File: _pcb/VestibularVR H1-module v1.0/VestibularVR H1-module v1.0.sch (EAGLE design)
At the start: 52 parts, among them IC1 FT232RL, IC2 74LVC1G07DBV, IC4 74LVC1G07DBV, IC5 74LVC1G07DBV, IC6 74LVC1G07DBV

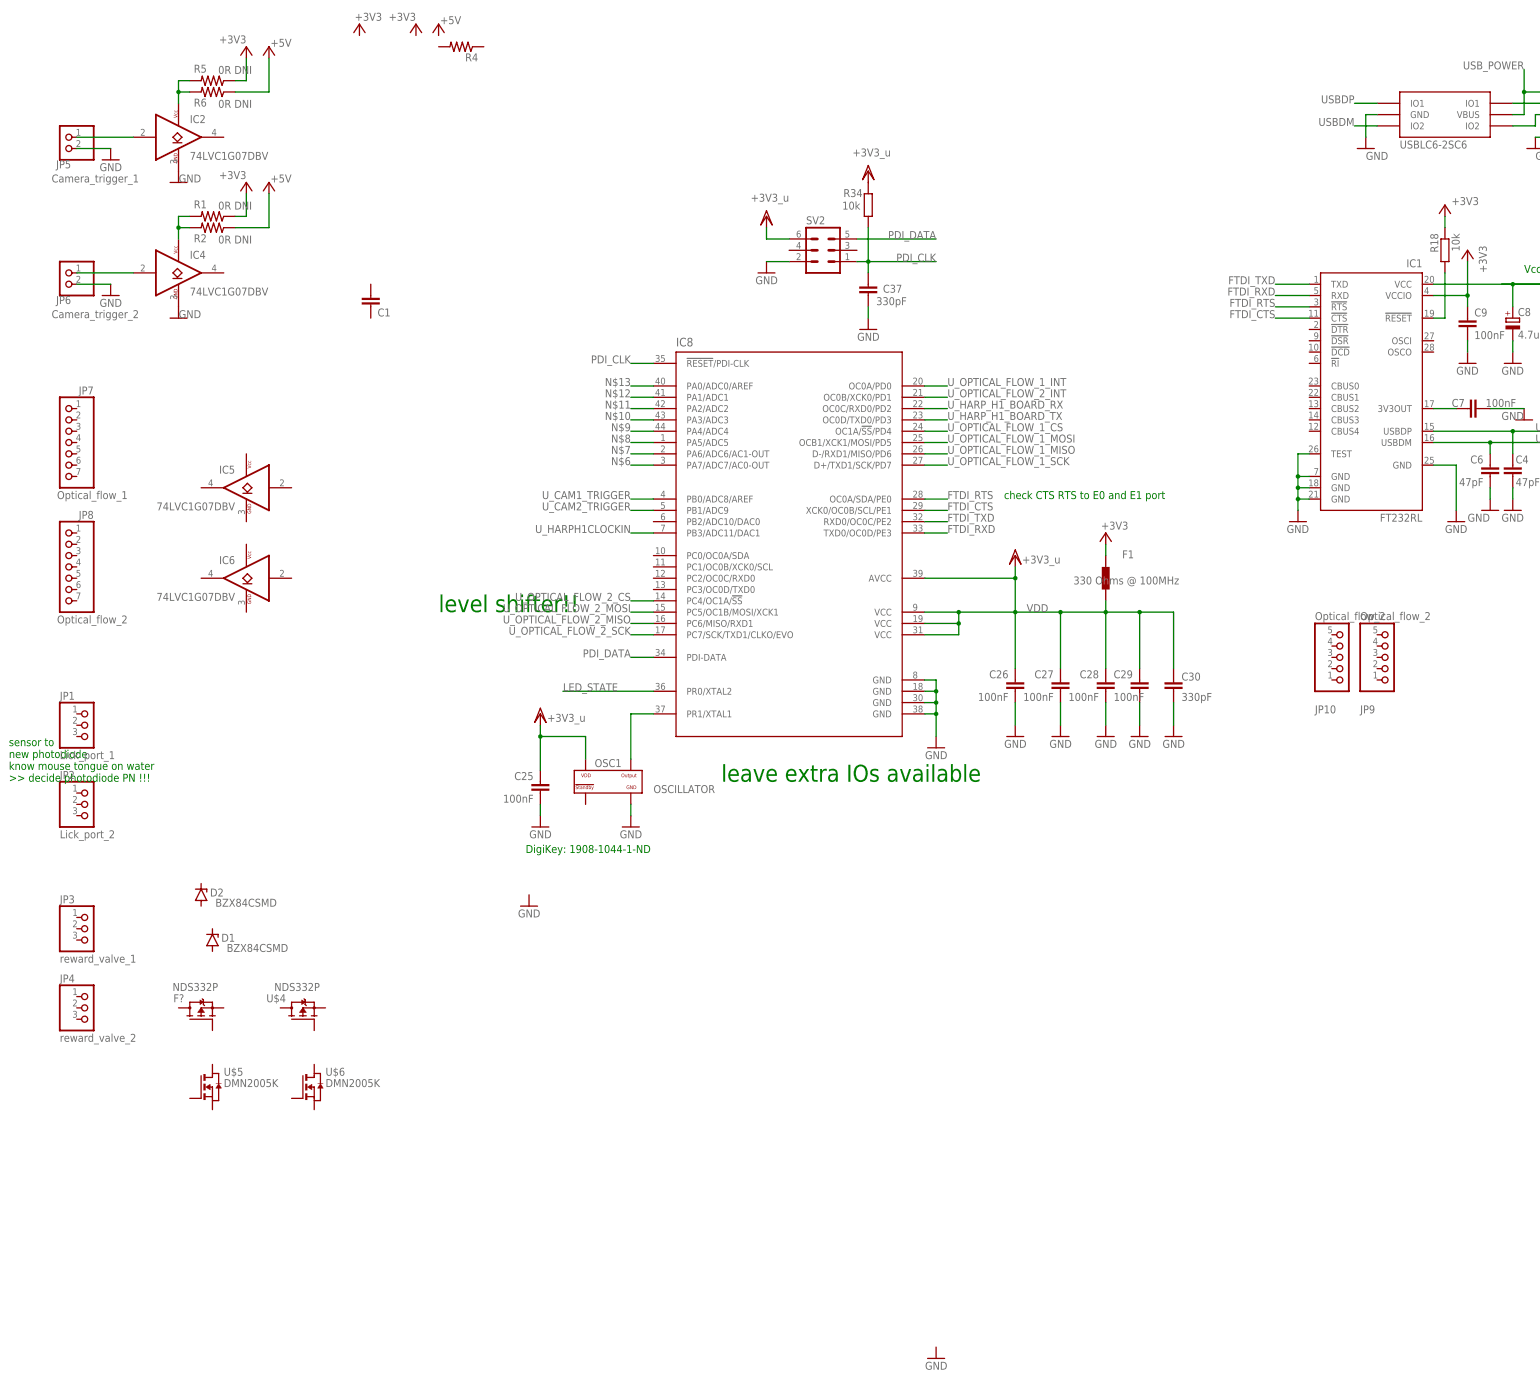
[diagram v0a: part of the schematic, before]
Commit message: pcb v1.0 developed
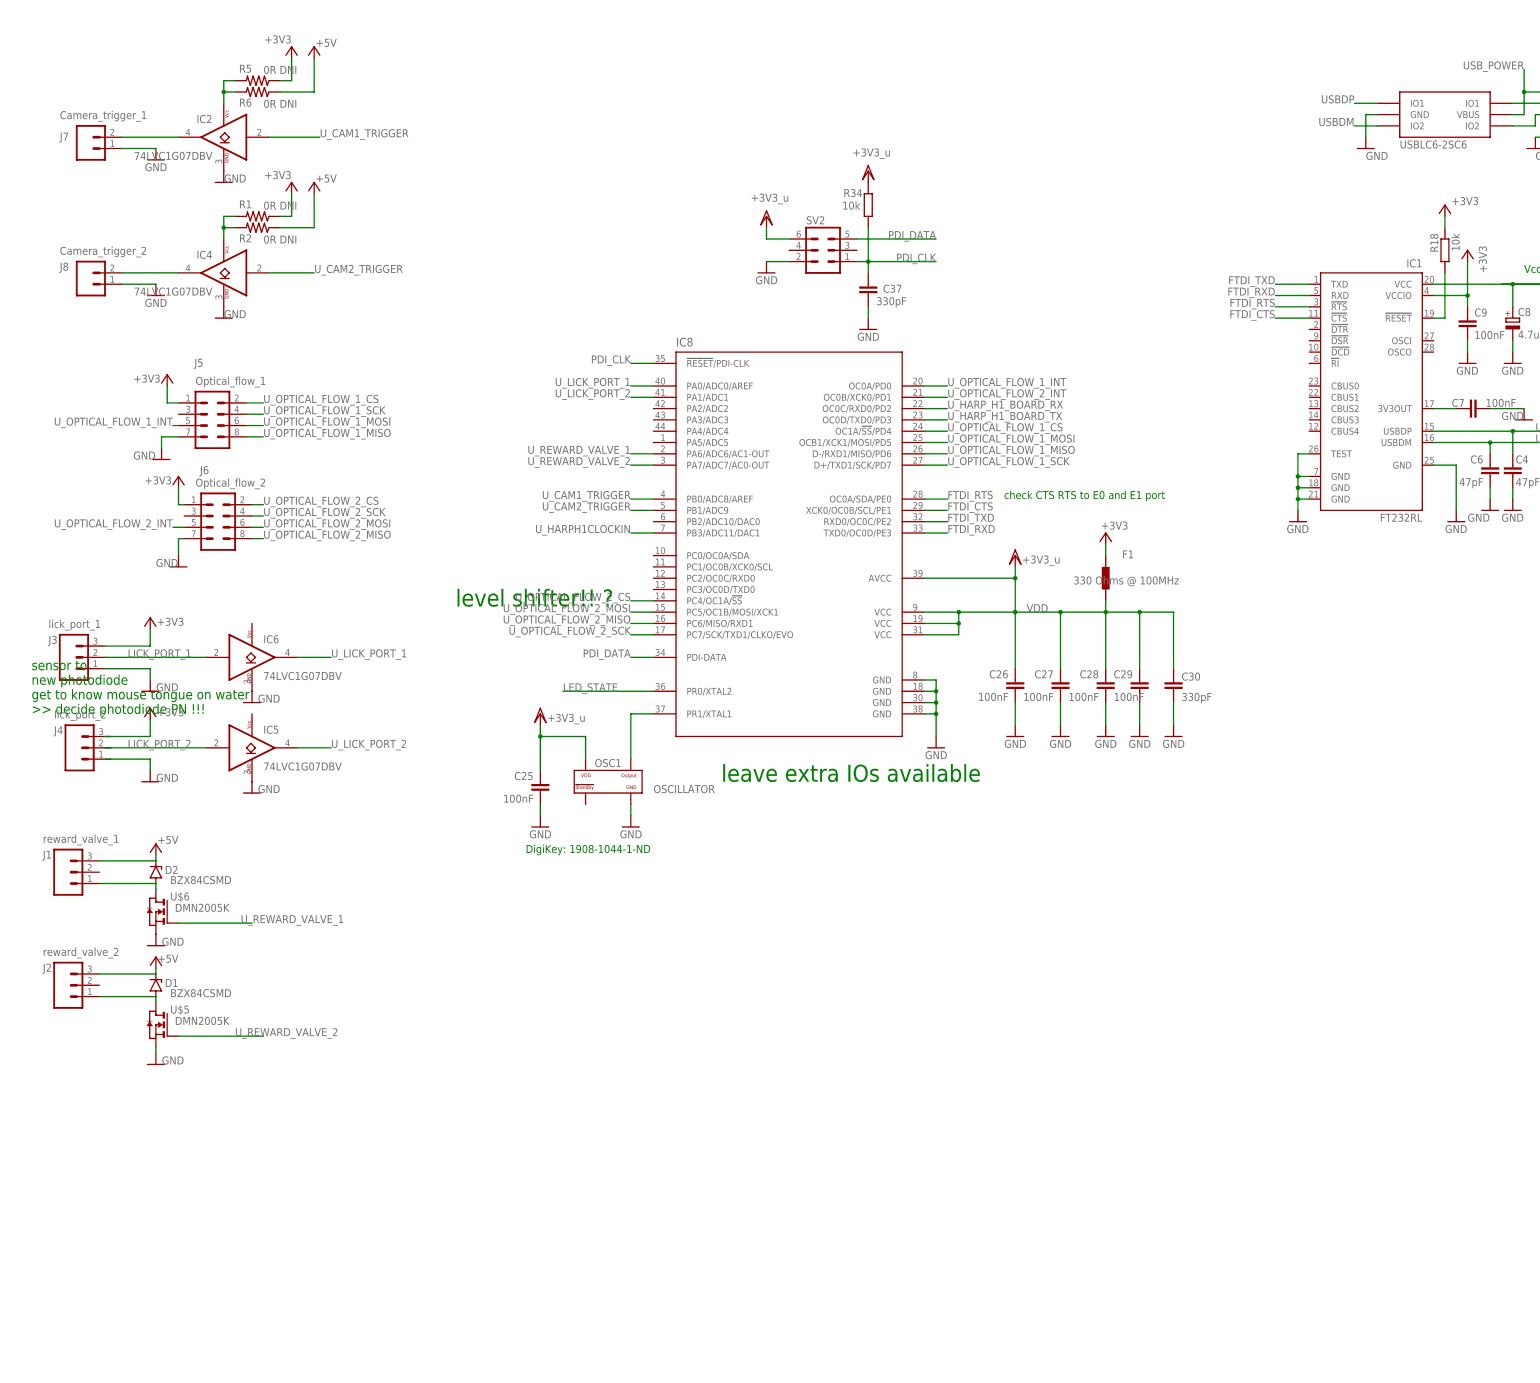
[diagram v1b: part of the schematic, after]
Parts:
- removed C1: (no value), rcl:C-EUC0402
- removed F?, U$4: NDS332P, VestibularVR H1-module v1.0:NDS332P
- removed JP1: Lick_port_1, pinhead:PINHD-1X3
- removed JP10, JP9: Optical_flow_2, pinhead:PINHD-1X5
- removed JP2: Lick_port_2, pinhead:PINHD-1X3
- removed JP3: reward_valve_1, pinhead:PINHD-1X3
- removed JP4: reward_valve_2, pinhead:PINHD-1X3
- removed JP5: Camera_trigger_1, pinhead:PINHD-1X2
- removed JP6: Camera_trigger_2, pinhead:PINHD-1X2
- removed JP7: Optical_flow_1, pinhead:PINHD-1X7
- removed JP8: Optical_flow_2, pinhead:PINHD-1X7
- removed R4: (no value), rcl:R-US_R0402
- added J1: reward_valve_1, SparkFun-Connectors:CONN_03JST-PTH-VERT
- added J2: reward_valve_2, SparkFun-Connectors:CONN_03JST-PTH-VERT
- added J3: lick_port_1, SparkFun-Connectors:CONN_03JST-PTH-VERT
- added J4: lick_port_2, SparkFun-Connectors:CONN_03JST-PTH-VERT
- added J5: Optical_flow_1, SparkFun-Connectors:CONN_04X2
- added J6: Optical_flow_2, SparkFun-Connectors:CONN_04X2
- added J7: Camera_trigger_1, SparkFun-Connectors:CONN_02POLAR
- added J8: Camera_trigger_2, SparkFun-Connectors:CONN_02POLAR
- renumbered U$3 to IC9
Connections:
- removed net N$10: IC8.PA3/ADC3
- removed net N$11: IC8.PA2/ADC2
- removed net N$12: IC8.PA1/ADC1
- removed net N$13: IC8.PA0/ADC0/AREF
- removed net N$7: IC8.PA6/ADC6/AC1-OUT
- removed net N$8: IC8.PA5/ADC5
- new net LICK_PORT_1: IC6.A, J3.2
- new net LICK_PORT_2: IC5.A, J4.2
- new net U_LICK_PORT_1: IC6.Y, IC8.PA0/ADC0/AREF
- new net U_LICK_PORT_2: IC5.Y, IC8.PA1/ADC1
- new net U_REWARD_VALVE_1: IC8.PA6/ADC6/AC1-OUT, U$6.G
- new net U_REWARD_VALVE_2: IC8.PA7/ADC7/AC0-OUT, U$5.G
- net +3V3: now also J3.3, J4.3, J5.1, J6.1
- net +5V: now also D1.C, D2.C, J1.3, J2.3
- net GND: now also IC5.GND, IC6.GND, J3.1, J4.1, J5.7, J6.7, J7.1, J8.1, U$5.S, U$6.S; no longer JP5.2, JP6.2
- net N$16: now also IC2.Y, J7.2; no longer IC2.A, JP5.1
- net N$4: now also IC4.Y, J8.2; no longer IC4.A, JP6.1
- net N$6: now also D1.A, J2.1, U$5.D; no longer IC8.PA7/ADC7/AC0-OUT
- net N$9: now also D2.A, J1.1, U$6.D; no longer IC8.PA4/ADC4
- net U_CAM1_TRIGGER: now also IC2.A
- net U_CAM2_TRIGGER: now also IC4.A
- net U_OPTICAL_FLOW_1_CS: now also J5.2
- net U_OPTICAL_FLOW_1_INT: now also J5.5
- net U_OPTICAL_FLOW_1_MISO: now also J5.8
- net U_OPTICAL_FLOW_1_MOSI: now also J5.6
- net U_OPTICAL_FLOW_1_SCK: now also J5.4
- net U_OPTICAL_FLOW_2_CS: now also J6.2
- net U_OPTICAL_FLOW_2_INT: now also J6.5
- net U_OPTICAL_FLOW_2_MISO: now also J6.8
- net U_OPTICAL_FLOW_2_MOSI: now also J6.6
- net U_OPTICAL_FLOW_2_SCK: now also J6.4
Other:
- note added: "level shifter!! ?"
- note added: "sensor to new photodiode get to know mouse tongue on water >> decide photodiode PN !!!"
- note removed: "level shifter!!"
- note removed: "sensor to new photodiode know mouse tongue on water >> decide photodiode PN !!!"
- moved on the sheet: D1, D2, IC2, IC4, IC5, IC6, R1, R2, R5, R6, U$5, U$6

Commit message: proceeding design VestibularVR H1
- Eagle version changed back to v.8.3.1
- proceeding design VestibularVR H1-module v1.0
- added Lick Sensor module v1.0
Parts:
- removed D2: BZX84CSMD, diode:BZX84CSMD
- removed IC9: USBLC6-2SC6, VestibularVR H1-module v1.0:USBLC6-2SC6
- removed J1: reward_valve_1, SparkFun-Connectors:CONN_03JST-PTH-VERT
- removed J2: reward_valve_2, SparkFun-Connectors:CONN_03JST-PTH-VERT
- removed J3: lick_port_1, SparkFun-Connectors:CONN_03JST-PTH-VERT
- removed J4: lick_port_2, SparkFun-Connectors:CONN_03JST-PTH-VERT
- removed J7: Camera_trigger_1, SparkFun-Connectors:CONN_02POLAR
- removed J8: Camera_trigger_2, SparkFun-Connectors:CONN_02POLAR
- removed OSC1: OSCILLATOR, harp camera controller:OSCILLATOR
- added C10, C11: 4.7uF, rcl:C-EUC0603
- added C12: 100nF, rcl:C-EUC0402
- added CAMERA_TRIGGER_1, CAMERA_TRIGGER_2, REWARD_VALVE_1, REWARD_VALVE_2: 22-23-2021, con-molex:22-23-2021
- added D4: BAT54, diode:BAT54
- added IC3: TLV70033DDCR, VestibularVR H1-module v1.0:TLV700XX
- added IC7: USBLC6-2SC6, VestibularVR H1-module v1.0:USBLC6-2SC6
- added LICK_PORT_1, LICK_PORT_2: 22-23-2031, con-molex:22-23-2031
- added R4, R7: 10k, rcl:R-US_R0402
- added U$2: OSCILLATOR, VestibularVR H1-module v1.0:OSCILLATOR
- added X7: 22-23-2051, con-molex:22-23-2051
- C8: device rcl:CPOL-EUA/3216-18W -> rcl:CPOL-EUA/3216-18R
- D1: value BZX84CSMD -> BAT54; device diode:BZX84CSMD -> diode:BAT54
- F1: device harp camera controller:BLM15HF0603 -> VestibularVR H1-module v1.0:BLM15HF0603
- IC8: value (none) -> ATXMEGA32A4U
- R18, R34: device rcl:R-EU_R0402 -> rcl:R-US_R0402
- SV2: value (none) -> PINHD-2X3; device con-lstb:MA03-2 -> Connector:PINHD-2X3
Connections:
- removed net N$15: C5.1, C8.+, IC1.VCC, L1.1
- removed net U_HARP_H1_BOARD_RX: IC8.OC0C/RXD0/PD2
- removed net U_HARP_H1_BOARD_TX: IC8.OC0D/TXD0/PD3
- removed net VDD: C25.1, C26.1, C27.1, C28.1, C29.1, C30.1, F1.1, IC8.AVCC, IC8.VCC@1, IC8.VCC@2, IC8.VCC@3, OSC1.VDD, R34.2, SV2.6
- new net +12V: X7-5.S
- new net +3V3_U: C25.1, C26.1, C27.1, C28.1, C29.1, C30.1, F1.1, IC8.AVCC, IC8.VCC@1, IC8.VCC@2, IC8.VCC@3, R34.2, SV2.6, U$2.VDD
- new net HARP_H1_BOARD_RX: IC8.OC0C/RXD0/PD2, X7-3.S
- new net HARP_H1_BOARD_TX: IC8.OC0D/TXD0/PD3, X7-4.S
- new net HARP_H1_CLOCK_IN: IC8.PC2/OC0C/RXD0, X7-2.S
- new net N$7: D4.C, REWARD_VALVE_2-2.S
- new net N$8: D1.C, REWARD_VALVE_1-2.S
- net +3V3: now also C11.1, C12.1, IC3.OUT, IC5.VCC, IC6.VCC, LICK_PORT_1-3.S, LICK_PORT_2-3.S; no longer J3.3, J4.3
- net +5V: now also C10.1, C5.1, C8.+, IC1.VCC, IC3.EN, IC3.IN, L1.1; no longer D1.C, D2.C, J1.3, J2.3
- net GND: now also C10.2, C11.2, C12.2, CAMERA_TRIGGER_1-1.S, CAMERA_TRIGGER_2-1.S, IC3.GND, IC7.GND, LICK_PORT_1-1.S, LICK_PORT_2-1.S, R4.1, R7.1, U$2.GND, X7-1.S; no longer IC9.GND, J3.1, J4.1, J7.1, J8.1, OSC1.GND
- net LICK_PORT_1: now also LICK_PORT_1-2.S; no longer J3.2
- net LICK_PORT_2: now also LICK_PORT_2-2.S; no longer J4.2
- net N$16: now also CAMERA_TRIGGER_1-2.S; no longer J7.2
- net N$2: now also IC7.IO2@1; no longer IC9.IO1@1
- net N$3: now also IC7.IO1@1; no longer IC9.IO2@1
- net N$4: now also CAMERA_TRIGGER_2-2.S; no longer J8.2
- net N$6: now also D4.A, REWARD_VALVE_2-1.S; no longer D1.A, J2.1
- net N$9: now also D1.A, REWARD_VALVE_1-1.S; no longer D2.A, J1.1
- net OSC2: now also U$2.OUTPUT; no longer OSC1.OUTPUT
- net USBDM: now also IC7.IO1@0; no longer IC9.IO2@0
- net USBDP: now also IC7.IO2@0; no longer IC9.IO1@0
- net USB_POWER: now also IC7.VBUS; no longer IC9.VBUS
- net U_CAM2_TRIGGER: now also IC8.OC0A/PD0; no longer IC8.PB1/ADC9
- net U_OPTICAL_FLOW_1_INT: no longer IC8.OC0A/PD0
- net U_OPTICAL_FLOW_2_INT: no longer IC8.OC0B/XCK0/PD1
- net U_REWARD_VALVE_1: now also R4.2
- net U_REWARD_VALVE_2: now also R7.2
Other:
- note added: "Camera_trigger_1"
- note added: "Camera_trigger_2"
- note added: "PAA5100JE Optical tracking - can be powered @ 3V3 oe 5V - line outputs level will depend of power"
- note added: "check CTS RTS to E0 and E1 port verificado com cammera controller - OK"
- note added: "lick sensor @3V3 GP1A57HRJ00F photointerrupter - design from FED3"
- note added: "lick_port_1"
- note added: "lick_port_2"
- note added: "main plug"
- note added: "reward_valve_1"
- note added: "reward_valve_2"
- note removed: "Vcc FTDI tb a net +5V ??"
- note removed: "check CTS RTS to E0 and E1 port"
- note removed: "level shifter!! ?"
- note removed: "sensor to new photodiode get to know mouse tongue on water >> decide photodiode PN !!!"
- moved on the sheet: C2, C25, C26, C27, C28, C29, C3, C30, C37, C4, C5, C6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
